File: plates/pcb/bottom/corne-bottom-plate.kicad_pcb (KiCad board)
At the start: 2 copper layers, 133.8 x 91.4 mm, 7 parts

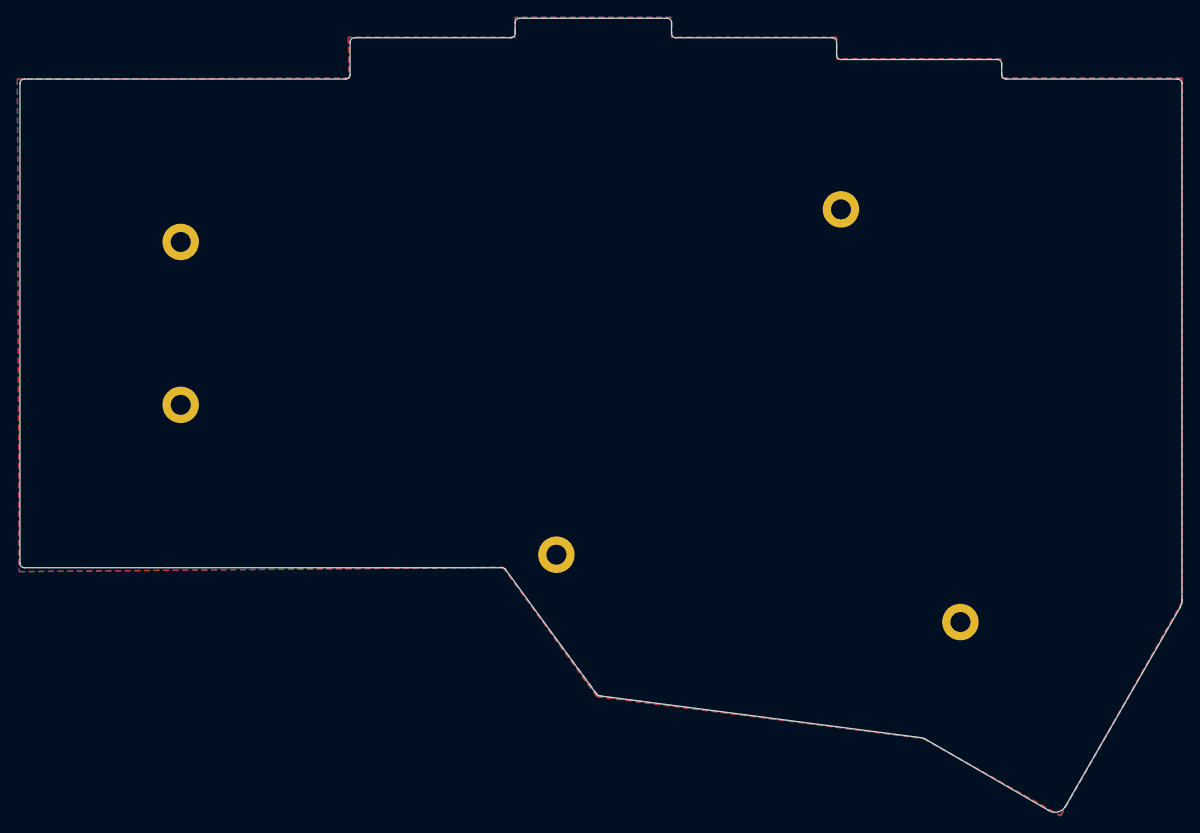
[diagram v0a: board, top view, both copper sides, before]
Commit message: plates
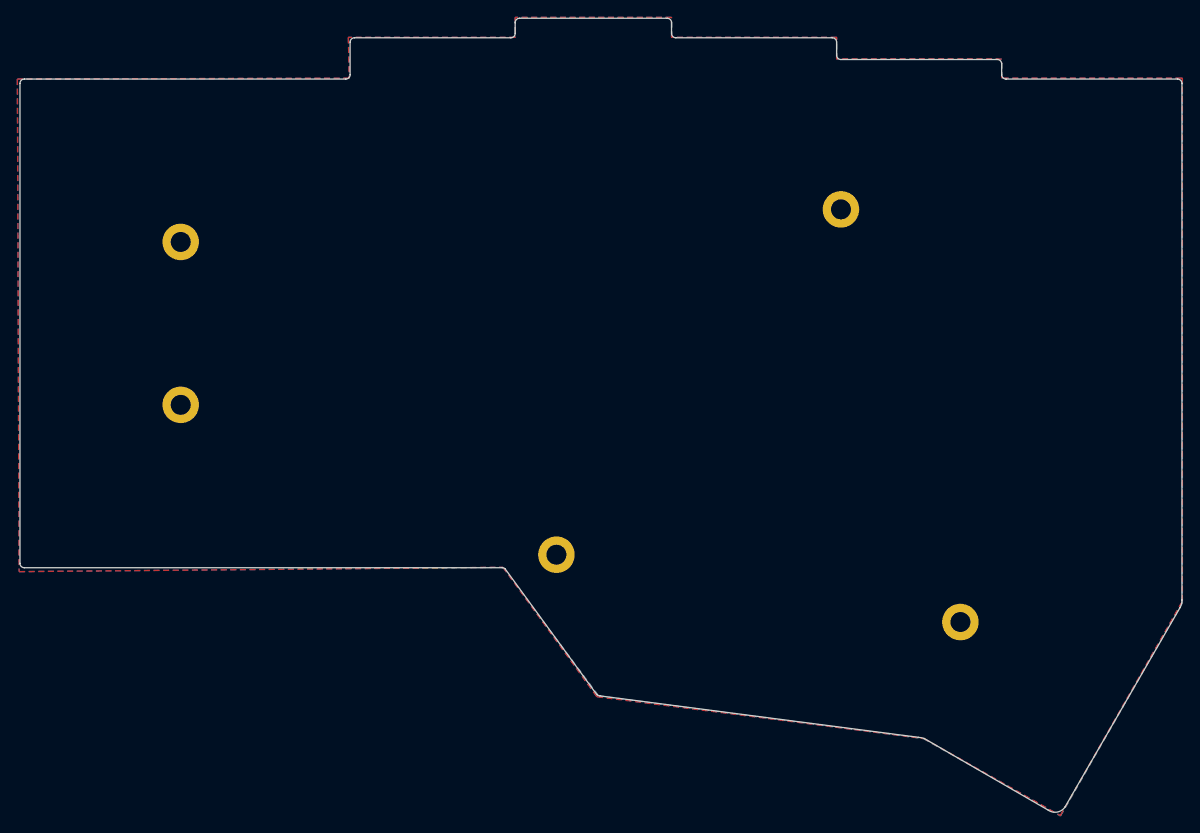
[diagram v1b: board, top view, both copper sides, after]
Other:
- net class Default removed
